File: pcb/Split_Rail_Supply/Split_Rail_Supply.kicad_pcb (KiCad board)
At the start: 2 copper layers, 17 parts, among them J1 Header_01x02_Wurth_61300211121, U1 TPS563206

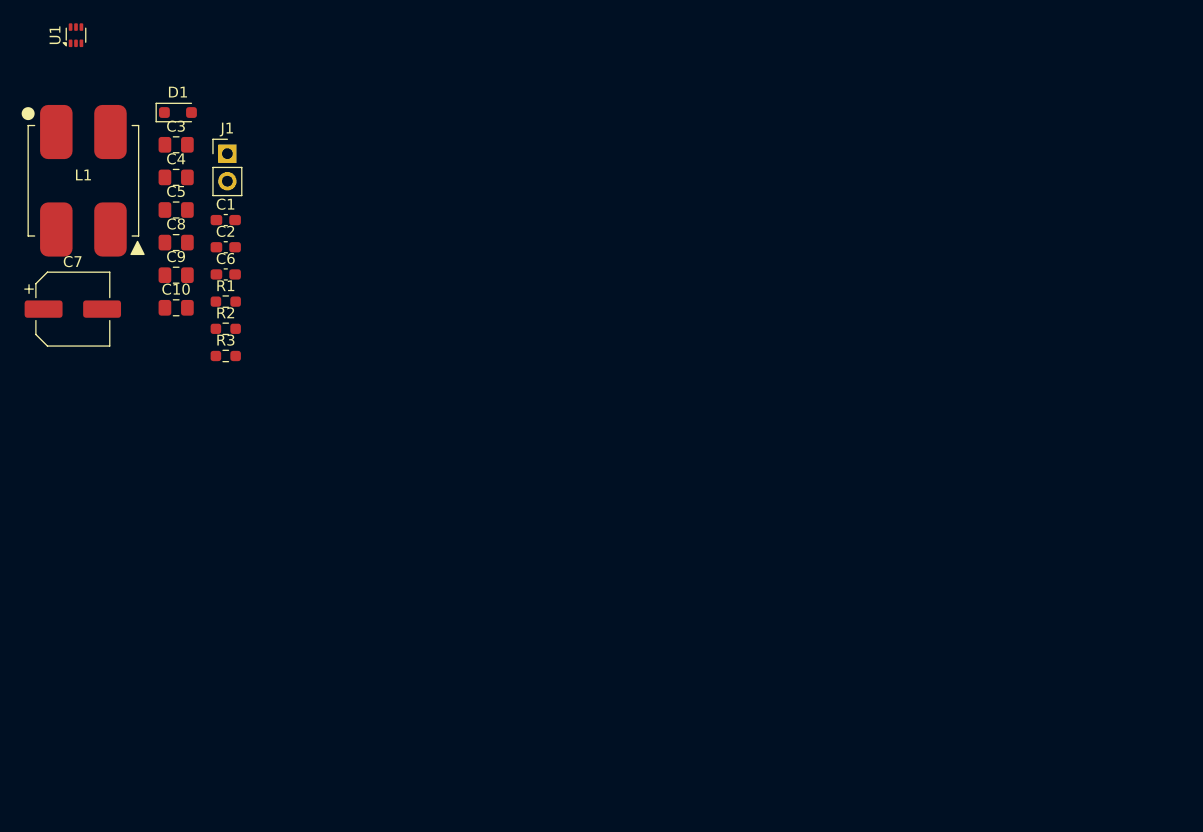
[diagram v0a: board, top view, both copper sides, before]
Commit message: Update SCH, PCB
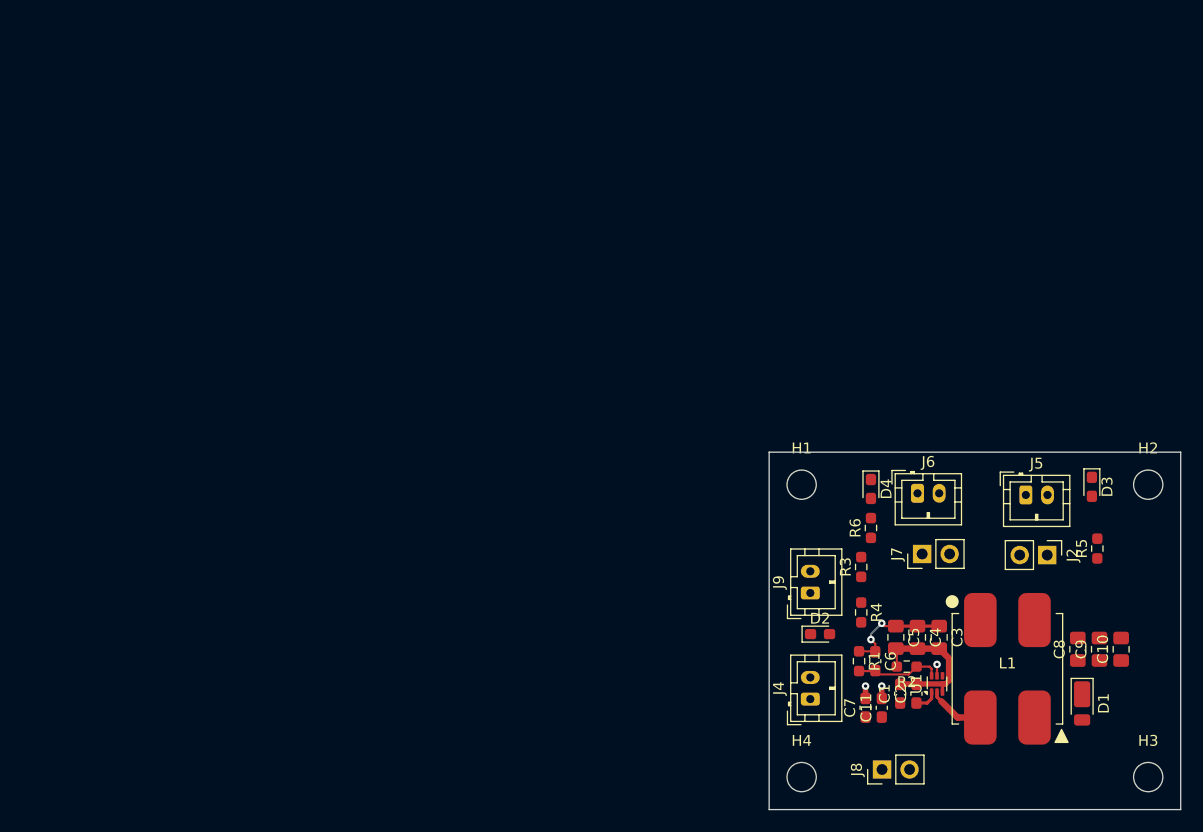
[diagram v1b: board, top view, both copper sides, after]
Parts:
- removed J1: Header_01x02_Wurth_61300211121, Connector_PinHeader_2.54mm:PinHeader_1x02_P2.54mm_Vertical
- added C11: 10uF,25V,X5R,0603, Capacitor_SMD:C_0603_1608Metric_Pad1.08x0.95mm_HandSolder, F.Cu at (138.4, 103.6)
- added D2: 150060GS75000, LED_SMD:LED_0603_1608Metric_Pad1.05x0.95mm_HandSolder, F.Cu at (132.7, 96.8)
- added D3: 150060GS75000, LED_SMD:LED_0603_1608Metric_Pad1.05x0.95mm_HandSolder, F.Cu at (157.8, 83.2)
- added D4: 150060GS75000, LED_SMD:LED_0603_1608Metric_Pad1.05x0.95mm_HandSolder, F.Cu at (137.4, 83.4)
- added H1: MountingHole, MountingHole:MountingHole_2.7mm_M2.5_DIN965, F.Cu at (131.0, 83.0)
- added H2: MountingHole, MountingHole:MountingHole_2.7mm_M2.5_DIN965, F.Cu at (163.0, 83.0)
- added H3: MountingHole, MountingHole:MountingHole_2.7mm_M2.5_DIN965, F.Cu at (163.0, 110.0)
- added H4: MountingHole, MountingHole:MountingHole_2.7mm_M2.5_DIN965, F.Cu at (131.0, 110.0)
- added J2: Header_01x02_Wurth_61300211121, Connector_PinHeader_2.54mm:PinHeader_1x02_P2.54mm_Vertical, F.Cu at (153.7, 89.5)
- added J4: JST_B2B-PH-K-x, Connector_JST:JST_PH_B2B-PH-K_1x02_P2.00mm_Vertical, F.Cu at (131.8, 102.8)
- added J5: JST_B2B-PH-K-x, Connector_JST:JST_PH_B2B-PH-K_1x02_P2.00mm_Vertical, F.Cu at (151.7, 84.0)
- added J6: JST_B2B-PH-K-x, Connector_JST:JST_PH_B2B-PH-K_1x02_P2.00mm_Vertical, F.Cu at (141.7, 83.8)
- added J7: Header_01x02_Wurth_61300211121, Connector_PinHeader_2.54mm:PinHeader_1x02_P2.54mm_Vertical, F.Cu at (142.1, 89.4)
- added J8: Header_01x02_Wurth_61300211121, Connector_PinHeader_2.54mm:PinHeader_1x02_P2.54mm_Vertical, F.Cu at (138.4, 109.3)
- added J9: JST_B2B-PH-K-x, Connector_JST:JST_PH_B2B-PH-K_1x02_P2.00mm_Vertical, F.Cu at (131.8, 93.0)
- added R4: 1k,0603, Resistor_SMD:R_0603_1608Metric_Pad0.98x0.95mm_HandSolder, F.Cu at (136.5, 94.8)
- added R5: 2k,0603, Resistor_SMD:R_0603_1608Metric_Pad0.98x0.95mm_HandSolder, F.Cu at (158.3, 88.9)
- added R6: 2k,0603, Resistor_SMD:R_0603_1608Metric_Pad0.98x0.95mm_HandSolder, F.Cu at (137.4, 87.0)
- C7: value 47uF,35V,Elec,6.6x6.6mm -> 10uF,25V,X5R,0603; footprint Capacitor_SMD:CP_Elec_6.3x7.7 -> Capacitor_SMD:C_0603_1608Metric_Pad1.08x0.95mm_HandSolder
- D1: value NSR0530HT1G -> DFLS230L-7; footprint Diode_SMD:D_SOD-323_HandSoldering -> Diode_SMD:D_PowerDI-123
- U1: value TPS563206 -> TPS564255
- moved D1 99.7 mm to (156.9, 103.2), turned to -90 degrees
- moved U1 99.5 mm to (143.5, 101.4)
- moved L1 96.5 mm to (150.0, 100.0)
- moved C10 92.8 mm to (160.5, 98.2), turned to 90 degrees
- moved C9 92.0 mm to (158.5, 98.2), turned to 90 degrees
- moved C8 91.3 mm to (156.5, 98.2), turned to 90 degrees
- moved C3 83.9 mm to (143.7, 97.1), turned to -90 degrees
- moved C7 81.9 mm to (136.9, 103.6), turned to 90 degrees
- moved C4 80.6 mm to (141.7, 97.1), turned to -90 degrees
- moved C5 77.3 mm to (139.7, 97.1), turned to -90 degrees
- moved C1 76.1 mm to (140.1, 102.3), turned to 90 degrees
- moved C2 75.9 mm to (141.6, 102.3), turned to 90 degrees
- moved R2 70.2 mm to (140.7, 99.8), turned to 180 degrees
- moved C6 69.8 mm to (137.8, 99.3), turned to -90 degrees
- moved R1 67.2 mm to (136.3, 99.3), turned to -90 degrees
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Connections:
- C6 pad 2: -Vout -> /FB
- L1 pad 1: Net-(U1-SW) -> GND
- L1 pad 2: GND -> Net-(U1-SW)
- L1 pad 3: GND -> Net-(D1-A)
- L1 pad 4: Net-(D1-A) -> GND
- R1 pad 2: -Vout -> /FB
- R2 pad 1: -Vout -> /FB
- U1 pad 6: -Vout -> /FB
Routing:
- net GND: track 0.00 -> 15.1 mm, vias 0 -> 4
- net -Vout: track 0.00 -> 14.8 mm
- net /FB: track 0.00 -> 7.90 mm
- net Net-(U1-SW): track 0.00 -> 5.24 mm
- net /Vin: track 0.00 -> 2.42 mm
- net Net-(J9-Pin_2): track 0.00 -> 1.05 mm, vias 0 -> 1
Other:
- board outline added: 38 x 33 mm
